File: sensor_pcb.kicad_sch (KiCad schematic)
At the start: 43 parts, among them J1 RTDSensor, J3 Conn_01x08, U1 MAX31865, U2 MIC5225, U3 74LVC125

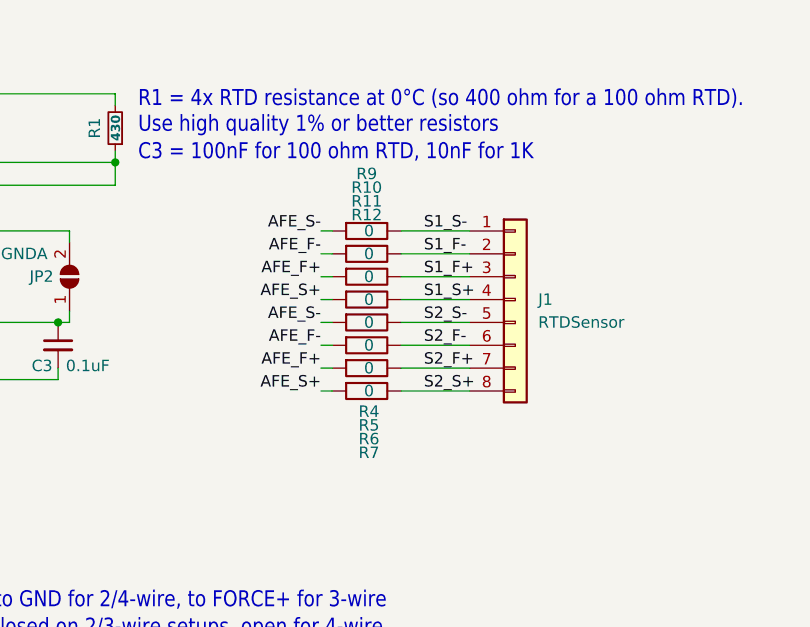
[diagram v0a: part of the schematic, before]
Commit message: Revision C of layout
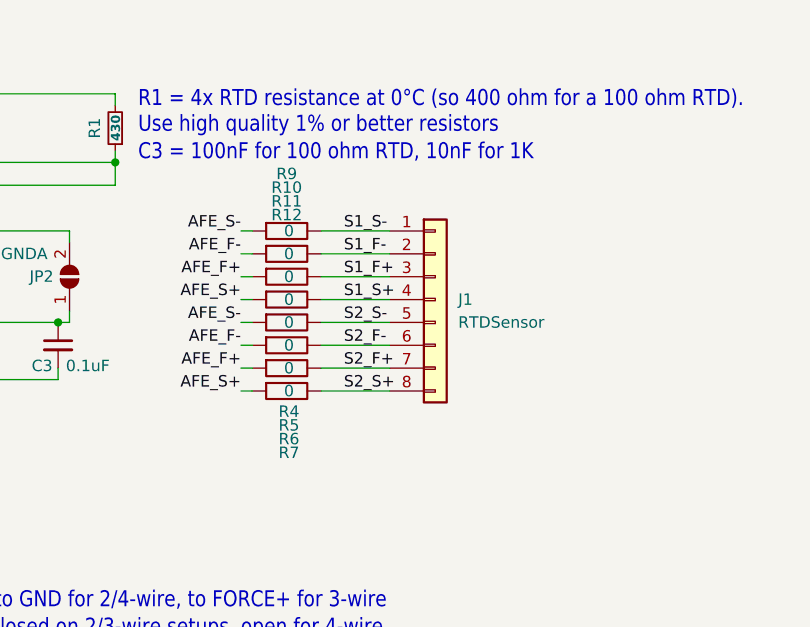
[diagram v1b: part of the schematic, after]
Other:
- moved on the sheet: J1, R10, R11, R12, R4, R5, R6, R7, R9
